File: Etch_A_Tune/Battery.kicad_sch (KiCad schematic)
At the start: 26 parts, among them U1 BQ297xy, U2 CSD16406Q3, U3 CSD16406Q3, U6 BQ25170DSGR

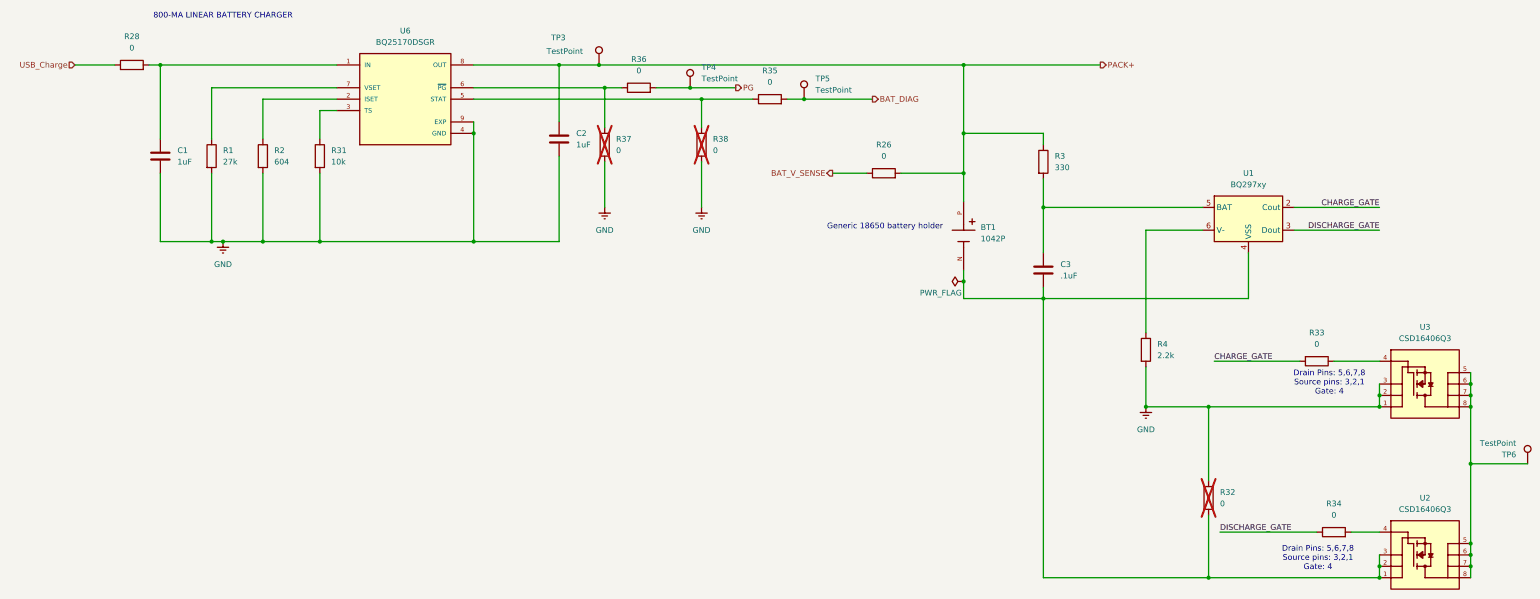
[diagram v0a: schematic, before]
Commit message: Another Update! :D
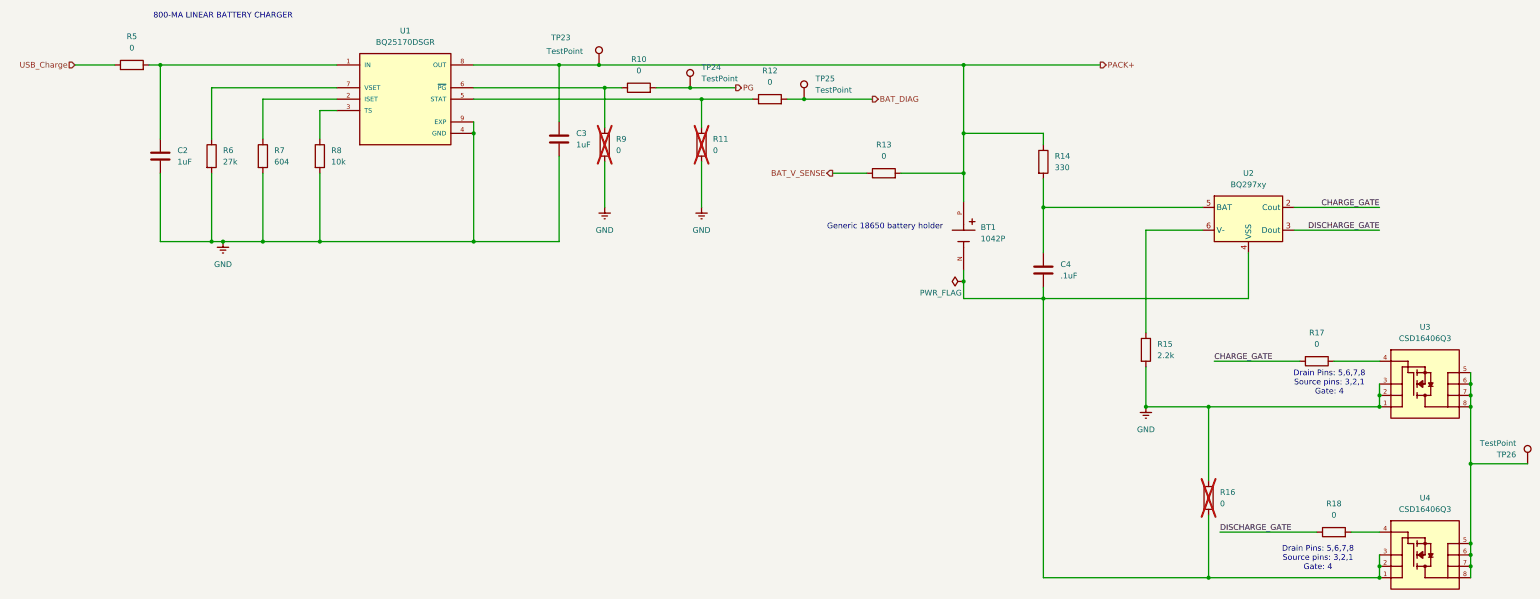
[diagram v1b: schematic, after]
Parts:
- renumbered C1 to C2, C2 to C3, C3 to C4, R36 to R10, R38 to R11, R35 to R12, R26 to R13, R3 to R14, R4 to R15, R32 to R16, R33 to R17, R34 to R18, R28 to R5, R1 to R6, R2 to R7, R31 to R8, R37 to R9, TP3 to TP23, TP4 to TP24, TP5 to TP25, TP6 to TP26, U6 to U1, U1 to U2, U2 to U4

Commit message: pdf docs
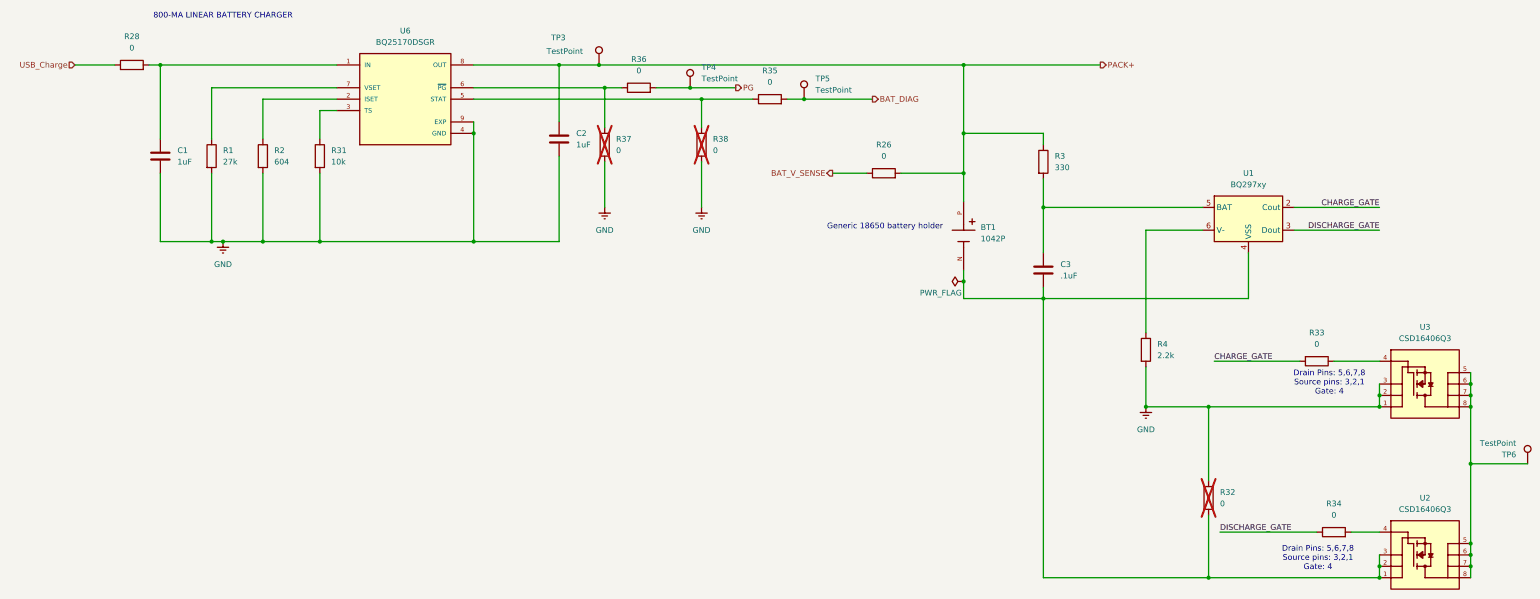
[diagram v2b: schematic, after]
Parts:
- renumbered C2 to C1, C3 to C2, C4 to C3, R6 to R1, R7 to R2, R13 to R26, R5 to R28, R14 to R3, R8 to R31, R16 to R32, R17 to R33, R18 to R34, R12 to R35, R10 to R36, R9 to R37, R11 to R38, R15 to R4, TP23 to TP3, TP24 to TP4, TP25 to TP5, TP26 to TP6, U2 to U1, U4 to U2, U1 to U6
